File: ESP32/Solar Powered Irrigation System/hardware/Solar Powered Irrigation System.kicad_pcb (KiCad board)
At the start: 2 copper layers, 69 parts, among them J1 GAS SENSOR, J12 +5V, J13 -5V, J2 SOIL SENSOR, J3 AM2301A, J4 OLED SCREEN, J5 GAS SENSOR, J7 USB_C Conn, J8 +IN, J9 -IN, Q1 IRLML6344, Q2 IRLML6344, Q3 UMH3N, SW2 RESET, SW3 FLASH, U1 AMS1117-3.3, U2 ESP32-WROOM, U3 LM2596S-3.3V, U4 LM2596S-3.3V, U5 CH340C, Y1 12MHz

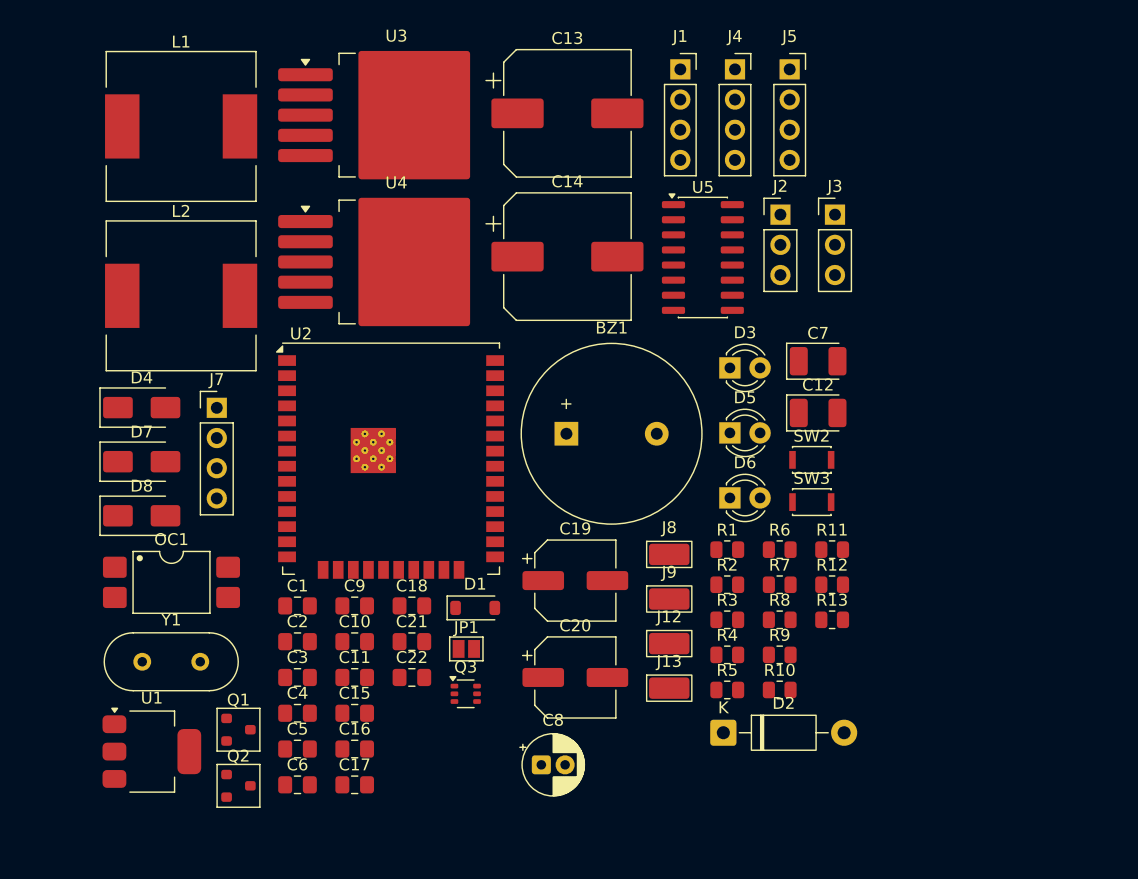
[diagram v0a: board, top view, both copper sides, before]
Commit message: Update from home
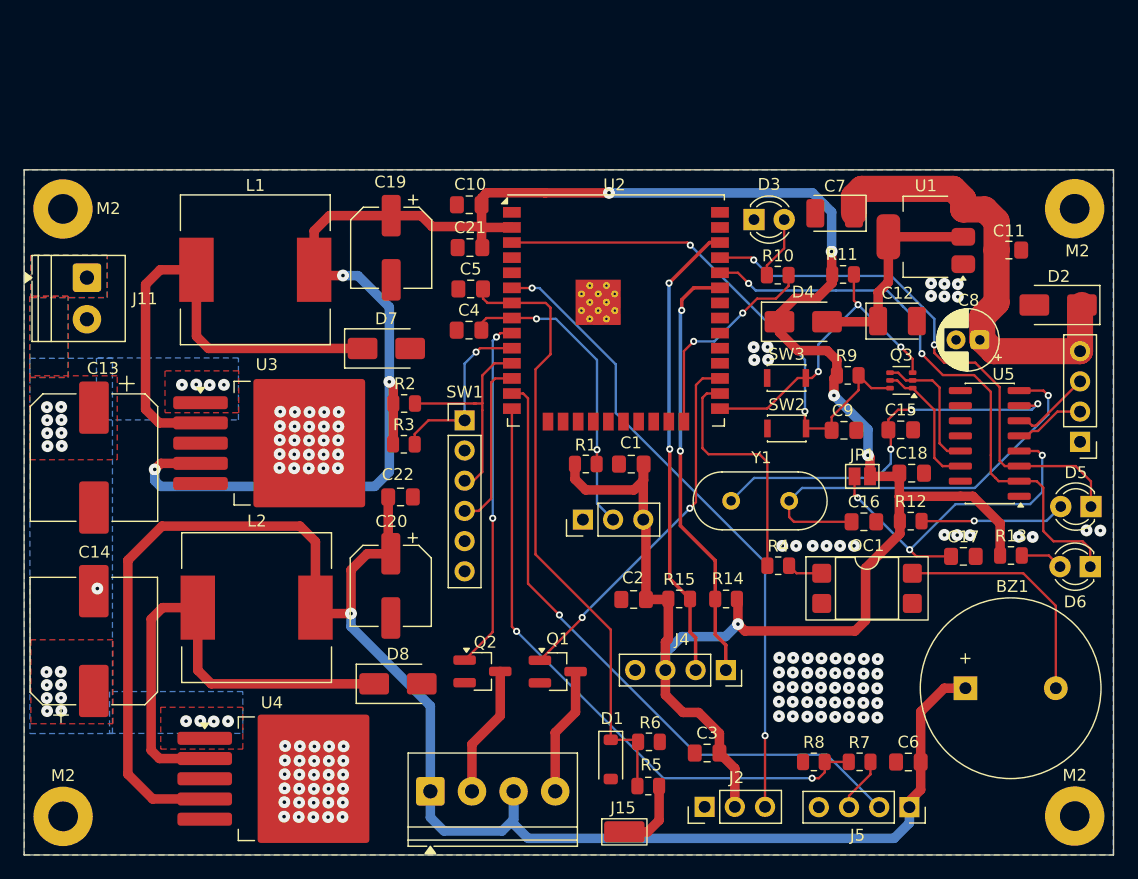
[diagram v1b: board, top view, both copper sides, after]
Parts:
- removed J12: +5V, TestPoint:TestPoint_Keystone_5015_Micro_Mini
- removed J13: -5V, TestPoint:TestPoint_Keystone_5015_Micro_Mini
- removed J8: +IN, TestPoint:TestPoint_Keystone_5015_Micro_Mini
- removed J9: -IN, TestPoint:TestPoint_Keystone_5015_Micro_Mini
- added J11: INPUT, TerminalBlock_Phoenix:TerminalBlock_Phoenix_PT-1,5-2-3.5-H_1x02_P3.50mm_Horizontal, F.Cu at (103.4, 88.3)
- added J15: BSEN, TestPoint:TestPoint_Keystone_5015_Micro_Mini, F.Cu at (148.6, 134.9)
- added M2: MountingHole_2.5mm_Pad, MountingHole:MountingHole_2.5mm_Pad, F.Cu at (186.5, 82.5)
- added M2: MountingHole_2.5mm_Pad, MountingHole:MountingHole_2.5mm_Pad, F.Cu at (186.5, 133.6)
- added M2: MountingHole_2.5mm_Pad, MountingHole:MountingHole_2.5mm_Pad, F.Cu at (101.4, 133.6)
- added M2: MountingHole_2.5mm_Pad, MountingHole:MountingHole_2.5mm_Pad, F.Cu at (101.4, 82.5)
- added R14: 10k, Resistor_SMD:R_0805_2012Metric, F.Cu at (157.2, 115.3)
- added R15: 10k, Resistor_SMD:R_0805_2012Metric, F.Cu at (153.2, 115.3)
- added SW1: RotaryEncoder, Connector_PinHeader_2.54mm:PinHeader_1x06_P2.54mm_Vertical, F.Cu at (135.2, 100.3)
- D2: footprint Diode_THT:D_DO-41_SOD81_P10.16mm_Horizontal -> Diode_SMD:D_SMA
- J1: value GAS SENSOR -> PUMP; footprint Connector_PinSocket_2.54mm:PinSocket_1x04_P2.54mm_Vertical -> TerminalBlock_Phoenix:TerminalBlock_Phoenix_PT-1,5-4-3.5-H_1x04_P3.50mm_Horizontal
- J5: value GAS SENSOR -> Ultra Sonic
- OC1: footprint PCM_Package_DIP_AKL:SMDIP-4_W9.53mm -> Package_DIP:DIP-4_W7.62mm_SMDSocket_SmallPads
- Q1, Q2: footprint PCM_Package_TO_SOT_SMD_AKL:SOT-23 -> Package_TO_SOT_SMD:SOT-23_Handsoldering
- moved U1 78.2 mm to (174.0, 84.9), turned to 180 degrees
- moved J7 72.7 mm to (186.9, 102.1), turned to 180 degrees
- moved C11 65.7 mm to (180.9, 86.0), turned to 180 degrees
- moved J1 64.3 mm to (132.3, 131.5)
- moved J5 62.9 mm to (172.6, 132.8), turned to -90 degrees
- moved OC1 58.5 mm to (169.0, 114.4)
- moved D4 56.1 mm to (163.7, 92.0)
- moved Y1 56.1 mm to (162.5, 107.1), turned to 180 degrees
- moved C17 54.7 mm to (177.1, 111.7), turned to 180 degrees
- moved C15 51.7 mm to (171.9, 101.1)
- moved C6 51.4 mm to (172.5, 129.0)
- moved C8 51.4 mm to (178.5, 93.5), turned to 180 degrees
- moved C14 51.3 mm to (104.0, 118.9), turned to 90 degrees
- moved J4 50.5 mm to (157.1, 121.3), turned to -90 degrees
- moved J2 50.2 mm to (155.4, 132.8), turned to 90 degrees
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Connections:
- net Net-(J7-Pin_2) renamed /+
- net Net-(J7-Pin_3) renamed /-
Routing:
- net +3.3V: track 0.00 -> 231.3 mm, vias 0 -> 8
- net +5V: track 0.00 -> 145.6 mm, vias 0 -> 1
- net /GPIO14: track 0.00 -> 54.5 mm, vias 0 -> 1
- net /GPIO34: track 0.00 -> 53.8 mm, vias 0 -> 2
- net /GPIO12: track 0.00 -> 53.0 mm, vias 0 -> 2
- net /GPIO35: track 0.00 -> 52.4 mm
- net /GPIO3/RX: track 0.00 -> 49.8 mm, vias 0 -> 2
- net /GPIO1/TX: track 0.00 -> 46.4 mm, vias 0 -> 2
- net /EN: track 0.00 -> 45.4 mm, vias 0 -> 2
- net Net-(D8-K): track 0.00 -> 40.7 mm
- net Net-(D7-K): track 0.00 -> 40.4 mm
- net /SCL: track 0.00 -> 39.2 mm, vias 0 -> 2
- net Net-(D2-K): track 0.00 -> 38.4 mm
- net /SDA: track 0.00 -> 36.4 mm, vias 0 -> 2
- net Net-(U5-Xo): track 0.00 -> 35.8 mm, vias 0 -> 1
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- added copper zone on B.Cu, net /VCC
- added copper zone on F.Cu, net /VCC
- added copper zone on B.Cu, net GND
- added copper zone on F.Cu, net GND
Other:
- board outline added: 91.6 x 57.6 mm
